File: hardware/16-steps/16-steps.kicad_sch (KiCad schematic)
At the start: 91 parts, among them J1 COLs 0-3, J2 ROWs / LEDs, J3 COLs 4-7, SW1 SW_Push, SW10 SW_Push, SW11 SW_Push, SW12 SW_Push, SW13 SW_Push, SW14 SW_Push, SW15 SW_Push, SW16 SW_Push, SW17 SW_Push, SW18 SW_Push, SW19 SW_Push, SW2 SW_Push, SW20 SW_Push, SW21 SW_Push, SW22 SW_Push, SW23 SW_Push, SW3 SW_Push, SW4 SW_Push, SW5 SW_Push, SW6 SW_Push, SW7 SW_Push, SW8 SW_Push, SW9 SW_Push

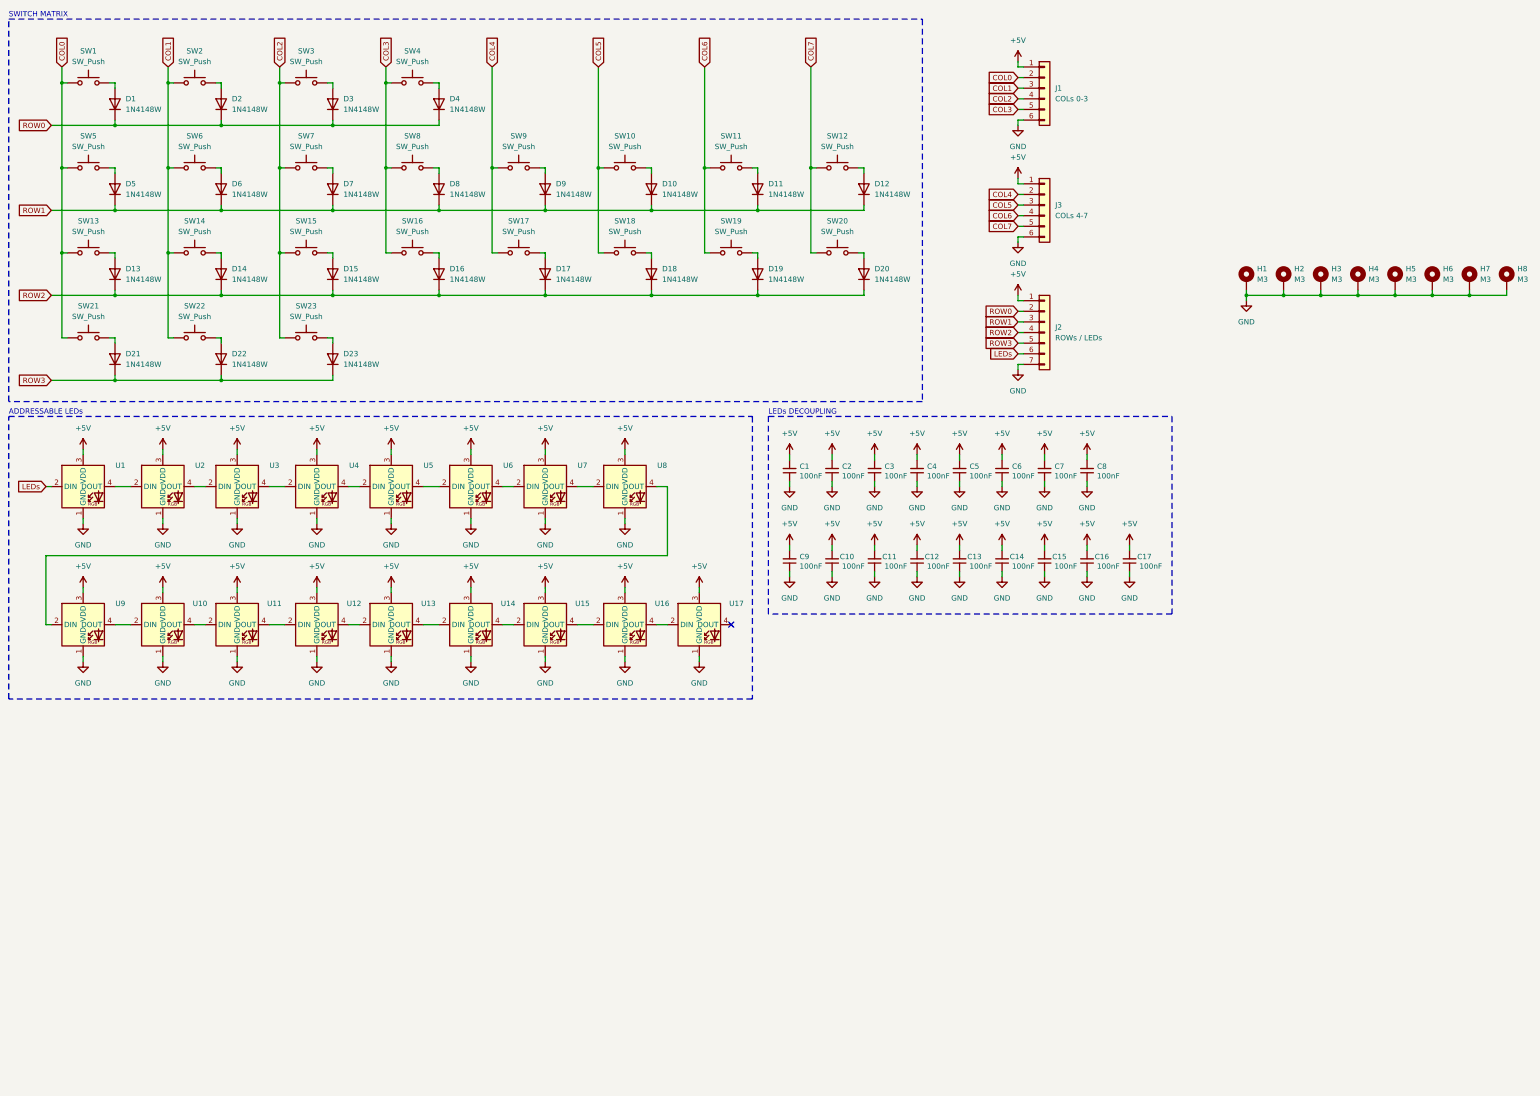
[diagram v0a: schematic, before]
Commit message: clean up, added pdf schematics
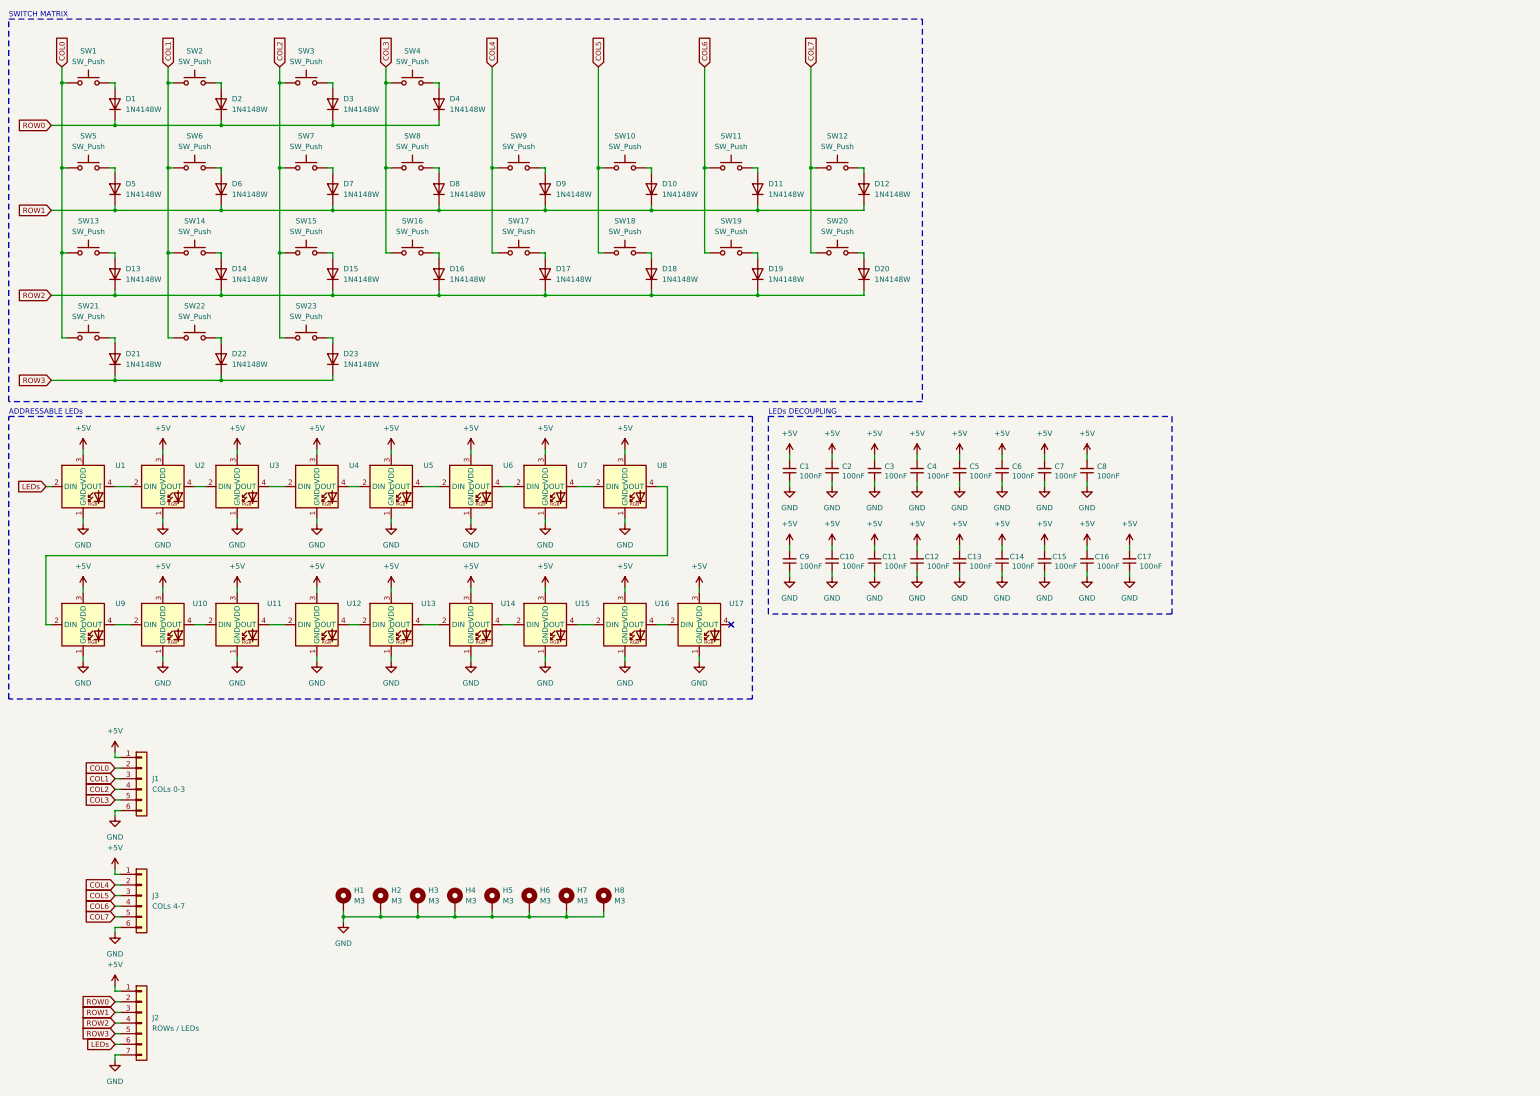
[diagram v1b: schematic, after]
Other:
- title: (none) -> Cherry MX 16-step Sequencer
- moved on the sheet: H1, H2, H3, H4, H5, H6, H7, H8, J1, J2, J3
